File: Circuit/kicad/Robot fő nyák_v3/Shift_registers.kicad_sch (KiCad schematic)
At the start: 18 parts, among them Q20 IRLML2502, Q21 IRLML2502, Q22 IRLML2502, Q23 IRLML2502, Q24 IRLML2502, Q25 IRLML2502, U53 MCP23S17_SO, U54 MCP23S17_SO

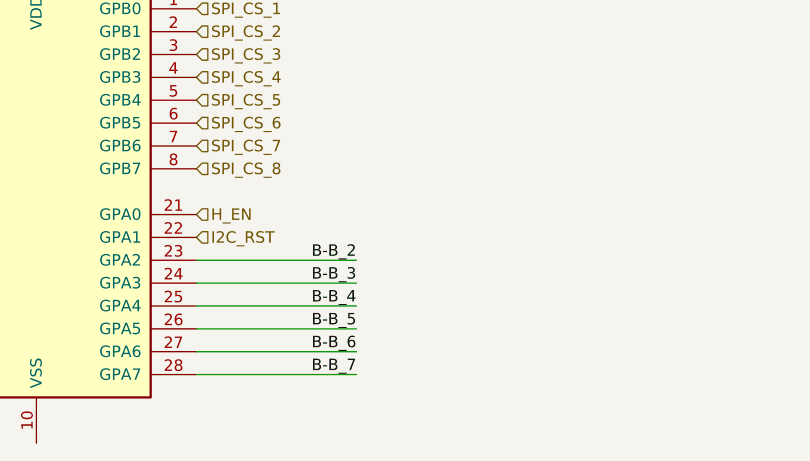
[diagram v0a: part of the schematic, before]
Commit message: kicad 2 panel_0.1
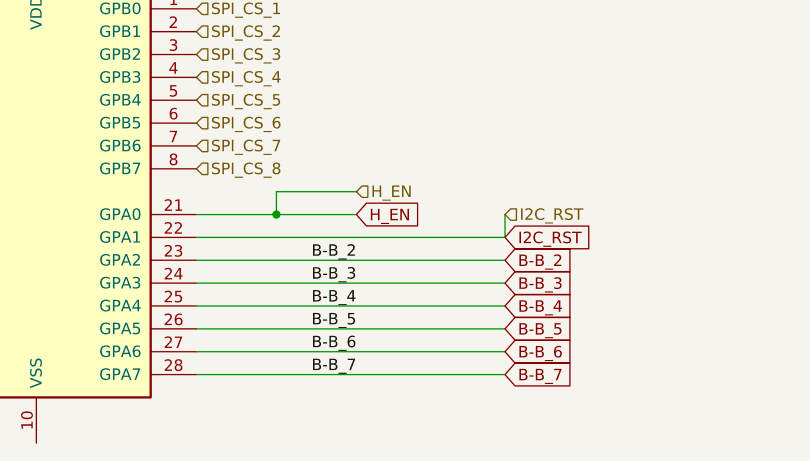
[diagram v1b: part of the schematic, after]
